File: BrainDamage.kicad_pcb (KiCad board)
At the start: 2 copper layers, 100 x 85 mm, 65 parts, among them CON1 AVR-ISP-10, IC1 ATMEGA328P-A, J1 TEST_2P, J10 Conn_01x02, J11 Conn_01x04, J12 Conn_01x04, J2 TEST_2P, J3 TEST_2P, J4 TEST_2P, J5 TEST_2P, J6 TEST_2P, J7 15A, J8 Bluetooth, J9 USB_OTG, P8 CONN_01X08, SW1 SW_PUSH, U1 PCA9685-TSSOP, U2 CH340G, U3 AP1117-50, X1 CRYSTAL_SMD, X2 CRYSTAL_SMD

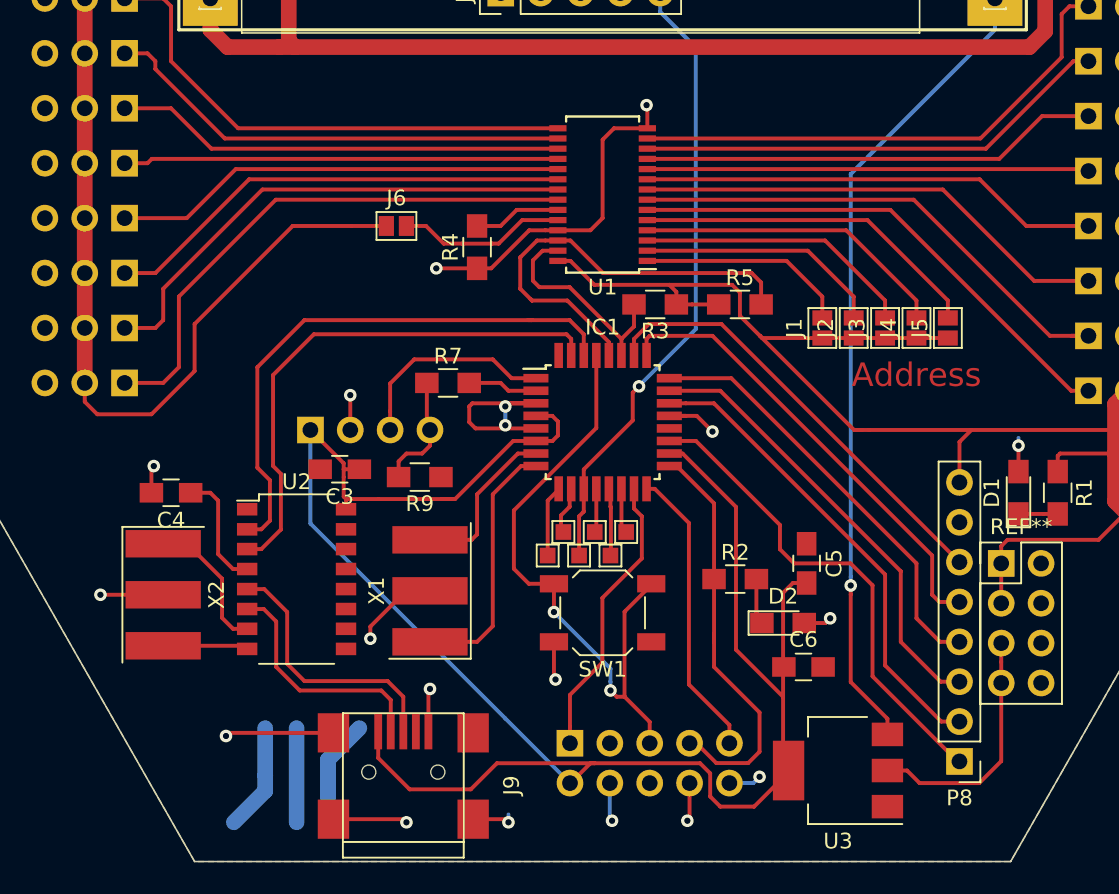
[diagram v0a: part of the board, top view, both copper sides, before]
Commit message: Add files via upload
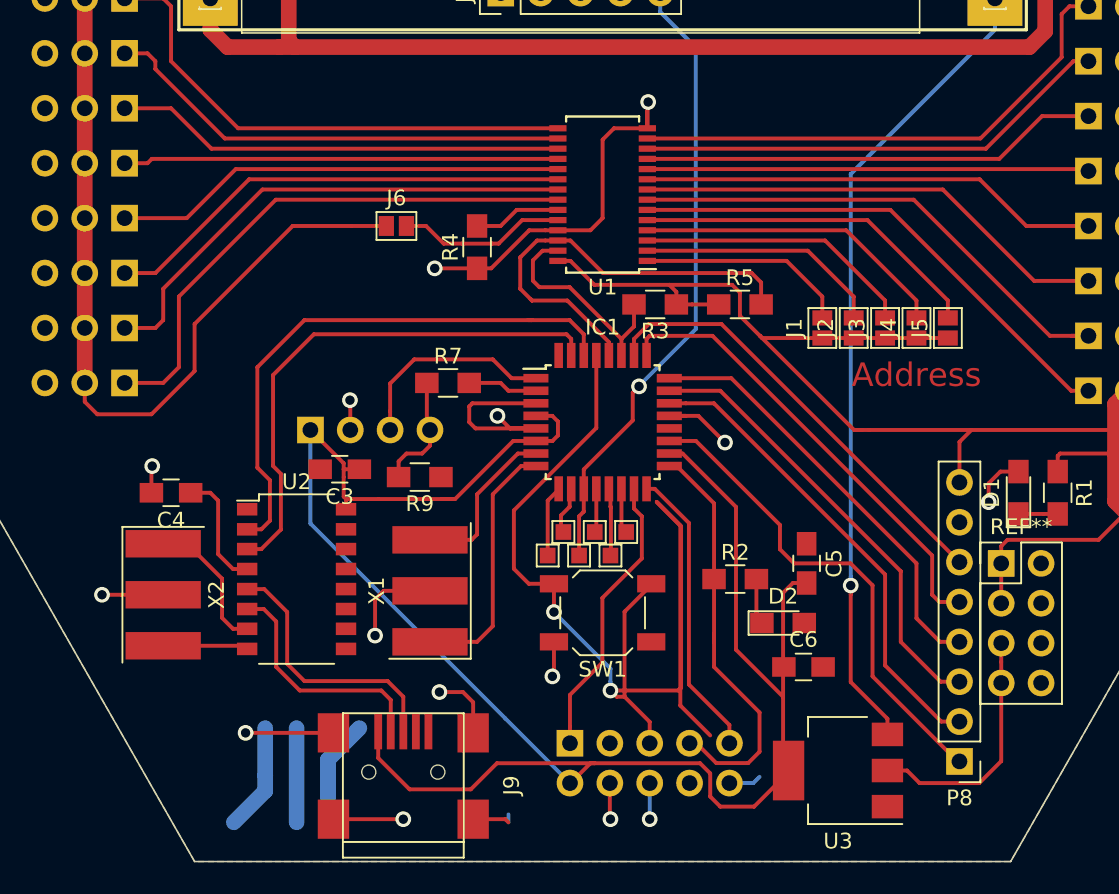
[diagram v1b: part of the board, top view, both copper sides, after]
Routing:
- net /RESET: track 39.6 -> 72.9 mm
- net GND: track 83.6 -> 85.4 mm, vias 19 -> 15
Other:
- net class Default: via_dia 0.8 -> 1; via_drill 0.4 -> 0.6
